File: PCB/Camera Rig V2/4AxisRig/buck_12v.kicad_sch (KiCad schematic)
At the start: 9 parts, among them U2 AN_SY8105

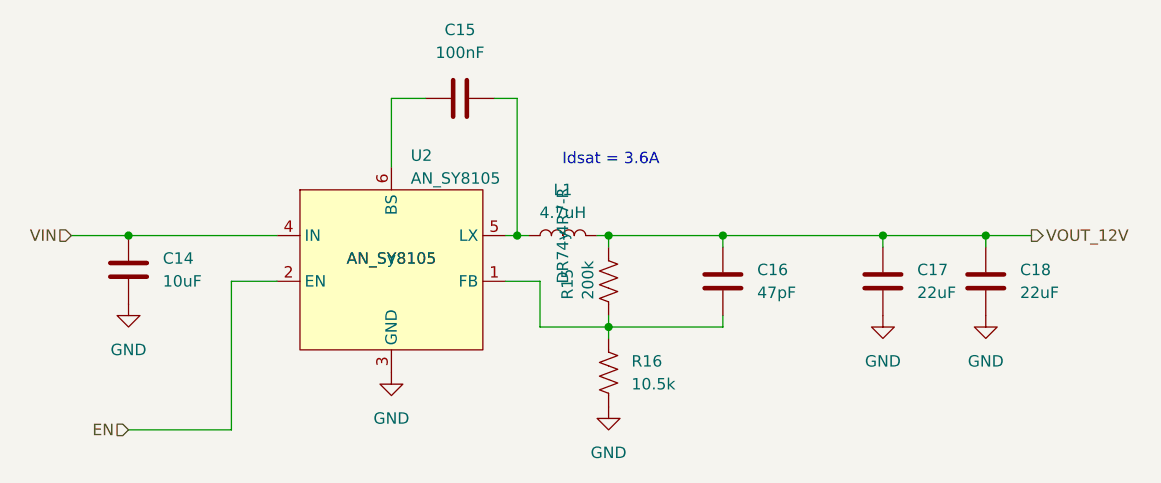
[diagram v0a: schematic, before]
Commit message: PCB V2 first draft
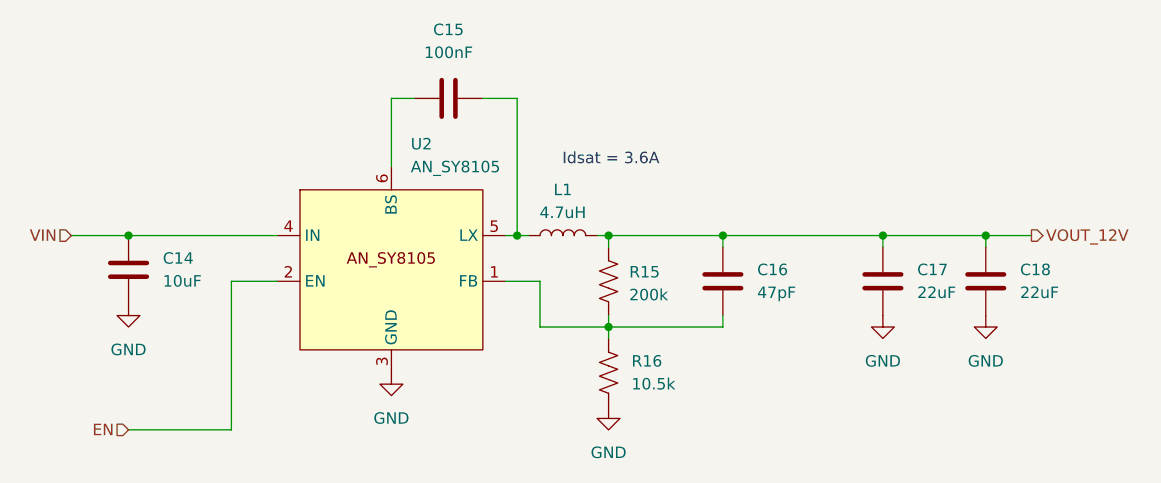
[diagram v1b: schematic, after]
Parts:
- C14, C15, C16: footprint (none) -> Capacitor_SMD:C_0603_1608Metric_Pad1.08x0.95mm_HandSolder
- C17, C18: footprint (none) -> Capacitor_SMD:C_1206_3216Metric_Pad1.33x1.80mm_HandSolder
- L1: footprint footprints:DR74 -> DR74-4R7-R:DR74; Unique FP y -> (none)
- U2: Unique FP y -> (none)
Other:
- moved on the sheet: C15
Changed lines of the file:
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@@
 	(wire
 		(pts
-			(xy 134.62 74.93) (xy 137.16 74.93)
+			(xy 133.35 74.93) (xy 137.16 74.93)
 		)
 		(stroke
@@
 	(wire
 		(pts
-			(xy 127 74.93) (xy 123.19 74.93)
+			(xy 125.73 74.93) (xy 123.19 74.93)
 		)
 		(stroke
@@
 			)
 		)
-		(property "Unique FP" ""
-			(at 147.32 105.41 0)
-			(effects
-				(font
-					(size 1.27 1.27)
-				)
-			)
-		)
 		(pin "2"
 		)
@@
 			)
 		)
-		(property "Footprint" ""
+		(property "Footprint" "Capacitor_SMD:C_0603_1608Metric_Pad1.08x0.95mm_HandSolder"
 			(at 94.9452 97.79 0)
 			(effects
@@
 		)
 		(property "Part Number" ""
-			(at 93.98 93.98 0)
-			(effects
-				(font
-					(size 1.27 1.27)
-				)
-			)
-		)
-		(property "Unique FP" ""
 			(at 93.98 93.98 0)
 			(effects
@@
 		(fields_autoplaced yes)
 		(property "Reference" "U2"
-			(at 125.3333 81.28 0)
+			(at 125.3333 80.01 0)
 			(effects
 				(font
@@
 		)
 		(property "Value" "AN_SY8105"
-			(at 125.3333 83.82 0)
+			(at 125.3333 82.55 0)
 			(effects
 				(font
@@
 					(size 1.27 1.27)
 				)
-			)
-		)
-		(property "Unique FP" "y"
-			(at 123.19 92.71 0)
-			(effects
-				(font
-					(size 1.27 1.27)
-				)
+				(hide yes)
 			)
 		)
@@
 			)
 		)
-		(property "Footprint" ""
+		(property "Footprint" "Capacitor_SMD:C_1206_3216Metric_Pad1.33x1.80mm_HandSolder"
 			(at 190.1952 99.06 0)
 			(effects
@@
 			)
 		)
-		(property "Datasheet" "~"
+		(property "Datasheet" "https://mm.digikey.com/Volume0/opasdata/d220001/medias/docus/506/TMK316BBJ226ML-T_SS.pdf"
 			(at 189.23 95.25 0)
 			(effects
@@
 		)
 		(property "Part Number" ""
-			(at 189.23 95.25 0)
-			(effects
-				(font
-					(size 1.27 1.27)
-				)
-			)
-		)
-		(property "Unique FP" ""
 			(at 189.23 95.25 0)
 			(effects
@@
 	(symbol
 		(lib_id "Device:C")
-		(at 130.81 74.93 270)
+		(at 129.54 74.93 270)
 		(unit 1)
 		(exclude_from_sim no)
@@
 		(fields_autoplaced yes)
 		(property "Reference" "C15"
-			(at 130.81 67.31 90)
+			(at 129.54 67.31 90)
 			(effects
 				(font
@@
 		)
 		(property "Value" "100nF"
-			(at 130.81 69.85 90)
-			(effects
-				(font
-					(size 1.27 1.27)
-				)
-			)
-		)
-		(property "Footprint" ""
-			(at 127 75.8952 0)
+			(at 129.54 69.85 90)
+			(effects
+				(font
+					(size 1.27 1.27)
+				)
+			)
+		)
+		(property "Footprint" "Capacitor_SMD:C_0603_1608Metric_Pad1.08x0.95mm_HandSolder"
+			(at 125.73 75.8952 0)
 			(effects
 				(font
@@
 		)
 		(property "Datasheet" "~"
-			(at 130.81 74.93 0)
+			(at 129.54 74.93 0)
 			(effects
 				(font
@@
 		)
 		(property "Description" "Unpolarized capacitor"
-			(at 130.81 74.93 0)
+			(at 129.54 74.93 0)
 			(effects
 				(font
@@
 		)
 		(property "Link" ""
-			(at 130.81 74.93 0)
+			(at 129.54 74.93 0)
 			(effects
 				(font
@@
 		)
 		(property "Part Number" ""
-			(at 130.81 74.93 0)
-			(effects
-				(font
-					(size 1.27 1.27)
-				)
-			)
-		)
-		(property "Unique FP" ""
-			(at 130.81 74.93 0)
+			(at 129.54 74.93 0)
 			(effects
 				(font
@@
 			)
 		)
-		(property "Footprint" "footprints:DR74"
+		(property "Footprint" "DR74-4R7-R:DR74"
 			(at 142.24 90.17 0)
 			(effects
@@
 					(size 1.27 1.27)
 				)
-			)
-		)
-		(property "Unique FP" "y"
-			(at 142.24 90.17 0)
-			(effects
-				(font
-					(size 1.27 1.27)
-				)
+				(hide yes)
 			)
 		)
@@
 			)
 		)
-		(property "Footprint" ""
+		(property "Footprint" "Capacitor_SMD:C_1206_3216Metric_Pad1.33x1.80mm_HandSolder"
 			(at 178.7652 99.06 0)
 			(effects
@@
 			)
 		)
-		(property "Datasheet" "~"
+		(property "Datasheet" "https://mm.digikey.com/Volume0/opasdata/d220001/medias/docus/506/TMK316BBJ226ML-T_SS.pdf"
 			(at 177.8 95.25 0)
 			(effects
@@
 		)
 		(property "Part Number" ""
-			(at 177.8 95.25 0)
-			(effects
-				(font
-					(size 1.27 1.27)
-				)
-			)
-		)
-		(property "Unique FP" ""
 			(at 177.8 95.25 0)
 			(effects
@@
 		(dnp no)
 		(property "Reference" "R15"
-			(at 142.748 97.282 90)
+			(at 149.606 94.234 0)
 			(effects
 				(font
@@
 		)
 		(property "Value" "200k"
-			(at 145.034 97.282 90)
+			(at 149.606 96.774 0)
 			(effects
 				(font
@@
 		)
 		(property "Part Number" ""
-			(at 147.32 95.25 0)
-			(effects
-				(font
-					(size 1.27 1.27)
-				)
-			)
-		)
-		(property "Unique FP" ""
 			(at 147.32 95.25 0)
 			(effects
@@
 			)
 		)
-		(property "Footprint" ""
+		(property "Footprint" "Capacitor_SMD:C_0603_1608Metric_Pad1.08x0.95mm_HandSolder"
 			(at 160.9852 99.06 0)
 			(effects
@@
 			(at 160.02 95.25 0)
 			(effects
-				(font
-					(size 1.27 1.27)
-				)
-			)
-		)
-		(property "Unique FP" ""
-			(at 160.02 95.25 0)
-			(effects
